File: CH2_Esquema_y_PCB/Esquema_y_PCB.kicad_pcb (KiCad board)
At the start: 2 copper layers, 140.1 x 79.8 mm, 44 parts, among them Q1 BC547, Q10 BC857, Q2 BC547, Q3 BC547, Q4 BC547, Q5 IRF9Z34N, Q7 BC547, Q9 BC857, U1 TL431LP, U2 LM358

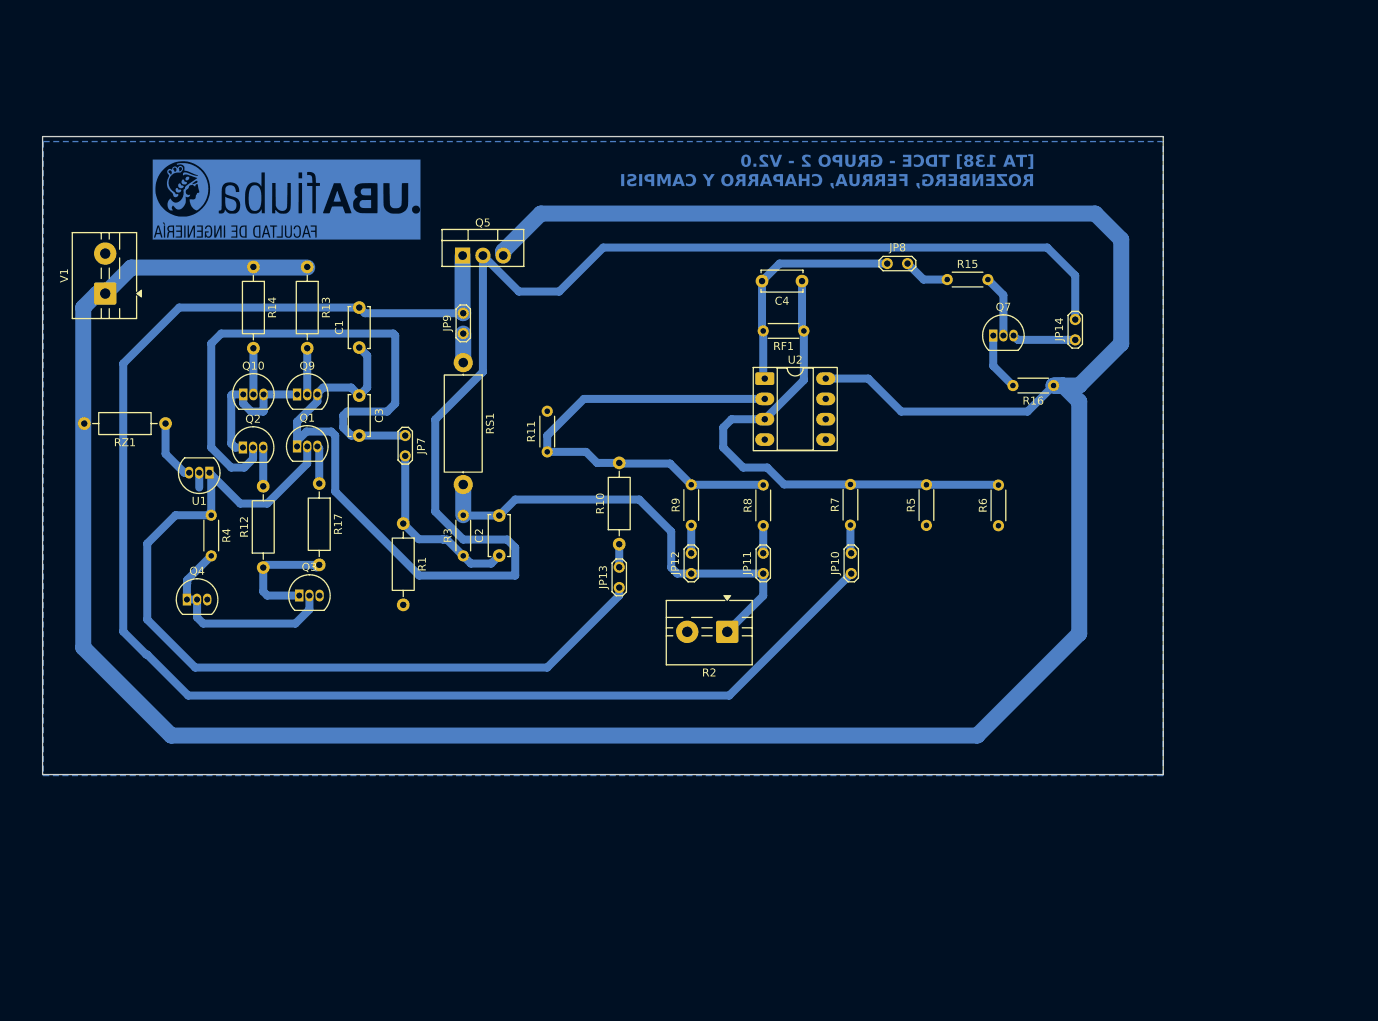
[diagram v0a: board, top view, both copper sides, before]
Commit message: Rehecho PCB
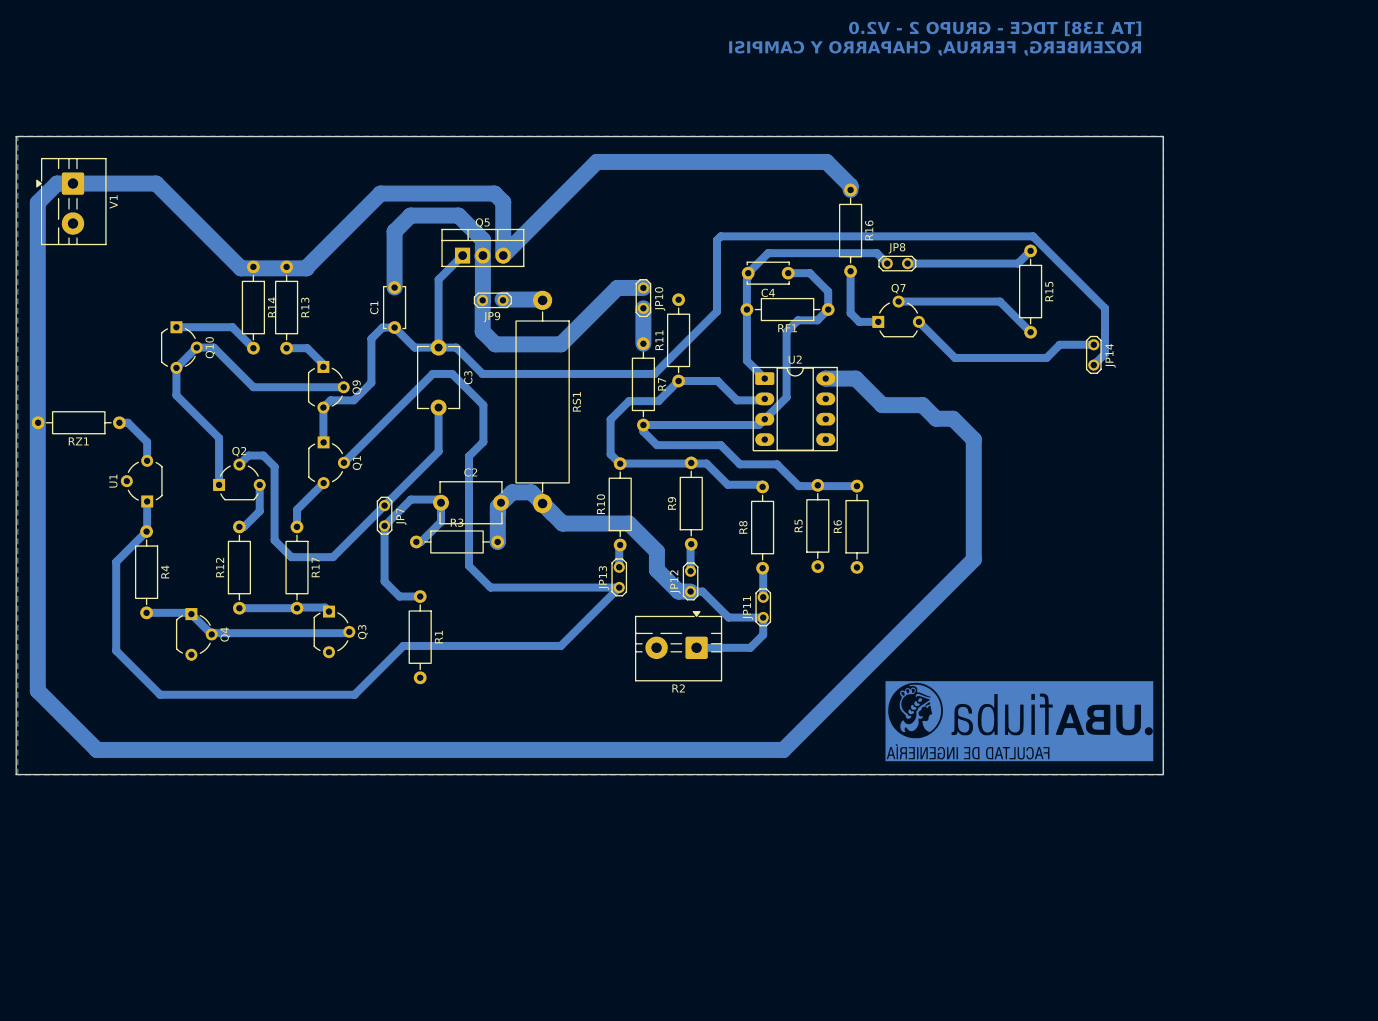
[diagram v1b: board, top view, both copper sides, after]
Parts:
- C2, C3: footprint Capacitor_THT:C_Disc_D5.0mm_W2.5mm_P5.00mm -> Capacitor_THT:C_Disc_D7.5mm_W5.0mm_P7.50mm
- Q1, Q10, Q2, Q3, Q4, Q7, Q9, U1: footprint Package_TO_SOT_THT:TO-92_Inline -> Package_TO_SOT_THT:TO-92_Wide
- R11, R15, R16, R3, R4, R5, R6, R7, R8, R9, RF1: footprint Resistor_THT:R_Axial_DIN0204_L3.6mm_D1.6mm_P5.08mm_Horizontal -> Resistor_THT:R_Axial_DIN0207_L6.3mm_D2.5mm_P10.16mm_Horizontal
- RS1: footprint Resistor_THT:R_Axial_DIN0414_L11.9mm_D4.5mm_P15.24mm_Horizontal -> Resistor_THT:R_Axial_Power_L20.0mm_W6.4mm_P25.40mm
- moved G*** 112.4 mm to (169.1, 108.2)
- moved JP10 44.2 mm to (122.1, 54.0), turned to -90 degrees
- moved R16 35.2 mm to (148.0, 41.8), turned to -90 degrees
- moved R7 34.4 mm to (122.1, 61.0), turned to -90 degrees
- moved R11 18.7 mm to (126.5, 65.7)
- moved R6 18.4 mm to (148.8, 89.0)
- moved R5 14.5 mm to (143.9, 88.9)
- moved Q7 14.5 mm to (151.5, 58.3)
- moved V1 14.3 mm to (50.8, 41.0), turned to -90 degrees
- moved RS1 12.6 mm to (109.5, 55.6)
- moved Q10 11.8 mm to (63.7, 59.0), turned to -90 degrees
- moved C3 11.6 mm to (96.5, 61.5)
- moved R15 11.0 mm to (170.5, 49.4), turned to -90 degrees
- moved C2 9.83 mm to (96.8, 80.9), turned to 0 degrees
- moved R1 9.36 mm to (94.2, 92.6)
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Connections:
- Q10 pad 1: Net-(Q10-B) -> Net-(Q10-E)
- Q10 pad 2: Net-(Q10-E) -> Net-(Q10-B)
- Q5 pad 1: /drain -> /gate
- Q5 pad 2: /gate -> /drain
- Q9 pad 1: Net-(Q10-B) -> Net-(Q9-E)
- Q9 pad 2: Net-(Q9-E) -> Net-(Q10-B)
- U2 pad 5: (no net) -> GND
- U2 pad 6: (no net) -> GND
- U2 pad 7: (no net) -> GND
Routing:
- net /drain: track 187.1 -> 55.4 mm
- net /gate: track 195.6 -> 148.4 mm
- net /in: track 109.0 -> 155.4 mm
- net VCC: track 376.3 -> 352.3 mm
- net Net-(JP7-A): track 70.0 -> 47.0 mm
- net Net-(Q10-B): track 19.6 -> 40.9 mm
- net Net-(JP14-A): track 7.93 -> 24.4 mm
- net Net-(U2A--): track 59.9 -> 47.4 mm
- net Net-(Q7-B): track 7.80 -> 18.1 mm
- net Net-(JP8-B): track 5.79 -> 16.0 mm
- net Net-(U2A-+): track 64.1 -> 72.7 mm
- net Net-(Q10-E): track 5.78 -> 10.9 mm
- net Net-(JP8-A): track 28.9 -> 33.1 mm
- net Net-(JP7-B): track 23.0 -> 27.3 mm
- net Net-(Q3-C): track 15.4 -> 11.4 mm
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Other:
- board size 140.1 x 79.8 mm -> 143.4 x 79.8 mm

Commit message: Reversion del PCB
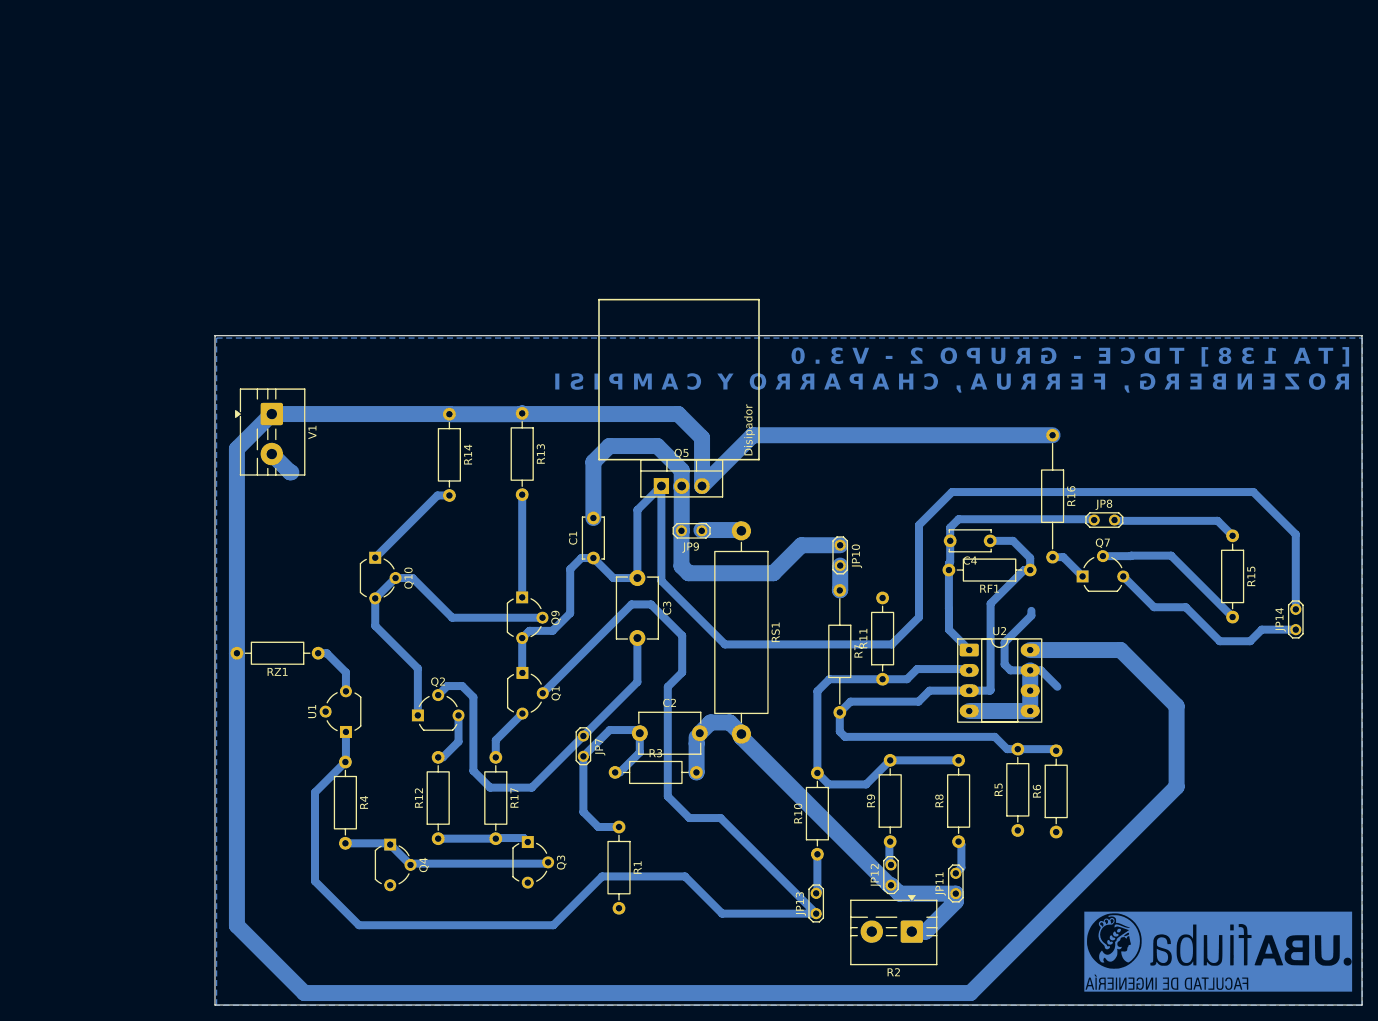
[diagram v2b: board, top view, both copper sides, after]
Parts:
- R16, R7: footprint Resistor_THT:R_Axial_DIN0207_L6.3mm_D2.5mm_P10.16mm_Horizontal -> Resistor_THT:R_Axial_DIN0207_L6.3mm_D2.5mm_P15.24mm_Horizontal
- moved JP13 47.6 mm to (143.7, 132.3)
- moved R10 45.8 mm to (143.8, 124.8)
- moved R11 45.2 mm to (152.0, 103.0)
- moved R9 44.7 mm to (152.9, 123.3)
- moved R2 44.5 mm to (155.7, 134.5)
- moved JP12 44.4 mm to (153.1, 128.7)
- moved JP14 43.7 mm to (203.7, 96.8), turned to 90 degrees
- moved R15 43.7 mm to (195.8, 85.0)
- moved U2 42.5 mm to (162.8, 99.3)
- moved JP11 42.1 mm to (161.2, 129.8)
- moved R8 42.1 mm to (161.5, 123.3)
- moved C4 41.9 mm to (165.4, 85.7)
- moved R6 41.4 mm to (173.7, 122.1)
- moved R5 41.4 mm to (168.9, 121.9)
- moved RF1 41.2 mm to (170.4, 89.3)
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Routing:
- net GND: track 0.00 -> 31.9 mm
- net VCC: track 352.3 -> 336.4 mm
- net /gate: track 148.4 -> 160.0 mm
- net Net-(Q9-E): track 5.76 -> 12.8 mm
- net /out: track 61.1 -> 55.2 mm
- net Net-(Q7-C): track 9.15 -> 4.75 mm
- net /in: track 155.4 -> 158.8 mm
- net Net-(U2A-+): track 72.7 -> 75.8 mm
- net Net-(U2A--): track 47.4 -> 49.9 mm
- net Net-(JP13-B): track 2.88 -> 5.27 mm
- net Net-(JP8-A): track 33.1 -> 34.9 mm
- net Net-(Q10-E): track 10.9 -> 12.5 mm
- net /drain: track 55.4 -> 53.9 mm
- net Net-(Q7-B): track 18.1 -> 19.4 mm
- net Net-(JP10-B): track 4.43 -> 3.13 mm
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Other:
- board size 143.4 x 79.8 mm -> 143.4 x 83.7 mm
- board text added: "Disipador"
- board text added: "[ T A 1 3 8 ] T D C E - G R U P O 2 - V 3 . 0 R O Z E N B E R G , F E R R U A , C H A P A R R O Y C A M P I S I"
- board text removed: "[TA 138] TDCE - GRUPO 2 - V2.0 ROZENBERG, FERRUA, CHAPARRO Y CAMPISI"
